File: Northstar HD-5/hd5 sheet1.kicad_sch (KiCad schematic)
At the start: 39 parts, among them Q1 2N3904, U1B1 26LS31, U1C1 74S10, U1D1 74S00, U1E1 50ns_Delay, U1F1 74S04, U1K1 LM393, U1L1 7438, U1M1 74LS374, U2D1 74LS175, U2E1 82S129, U2F1 74S174, U2J1 74LS393, U2K1 74LS393, U2L1 2114, U2M1 2114, U3K1 74LS164, U3L1 74LS374, U3M1 74LS166, U4J1 74LS04, U4K1 74LS244, U4L1 74LS244, U4M1 74LS244, U5L1 74LS138, U5M1 74LS138

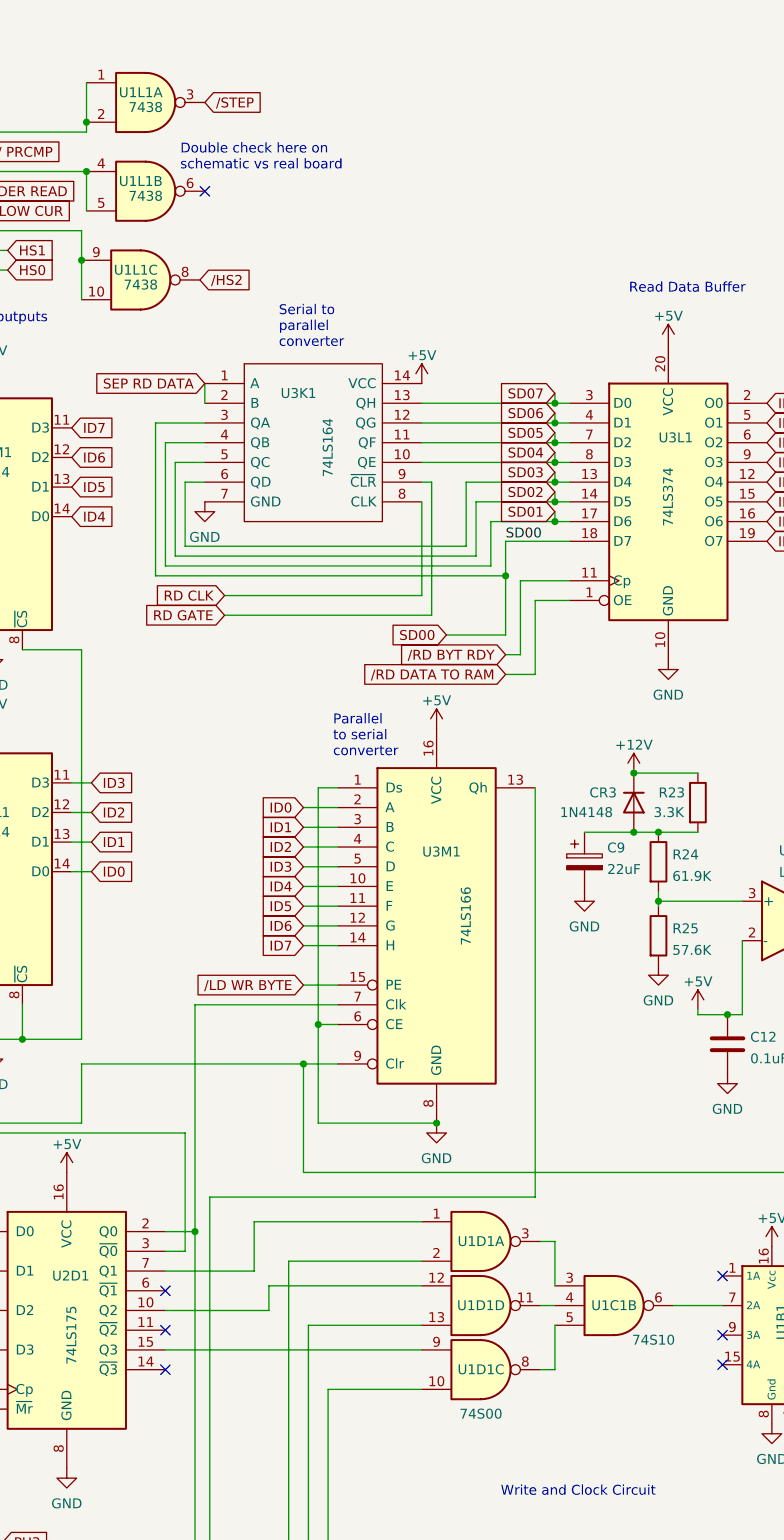
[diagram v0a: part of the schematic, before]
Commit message: small updates to boards
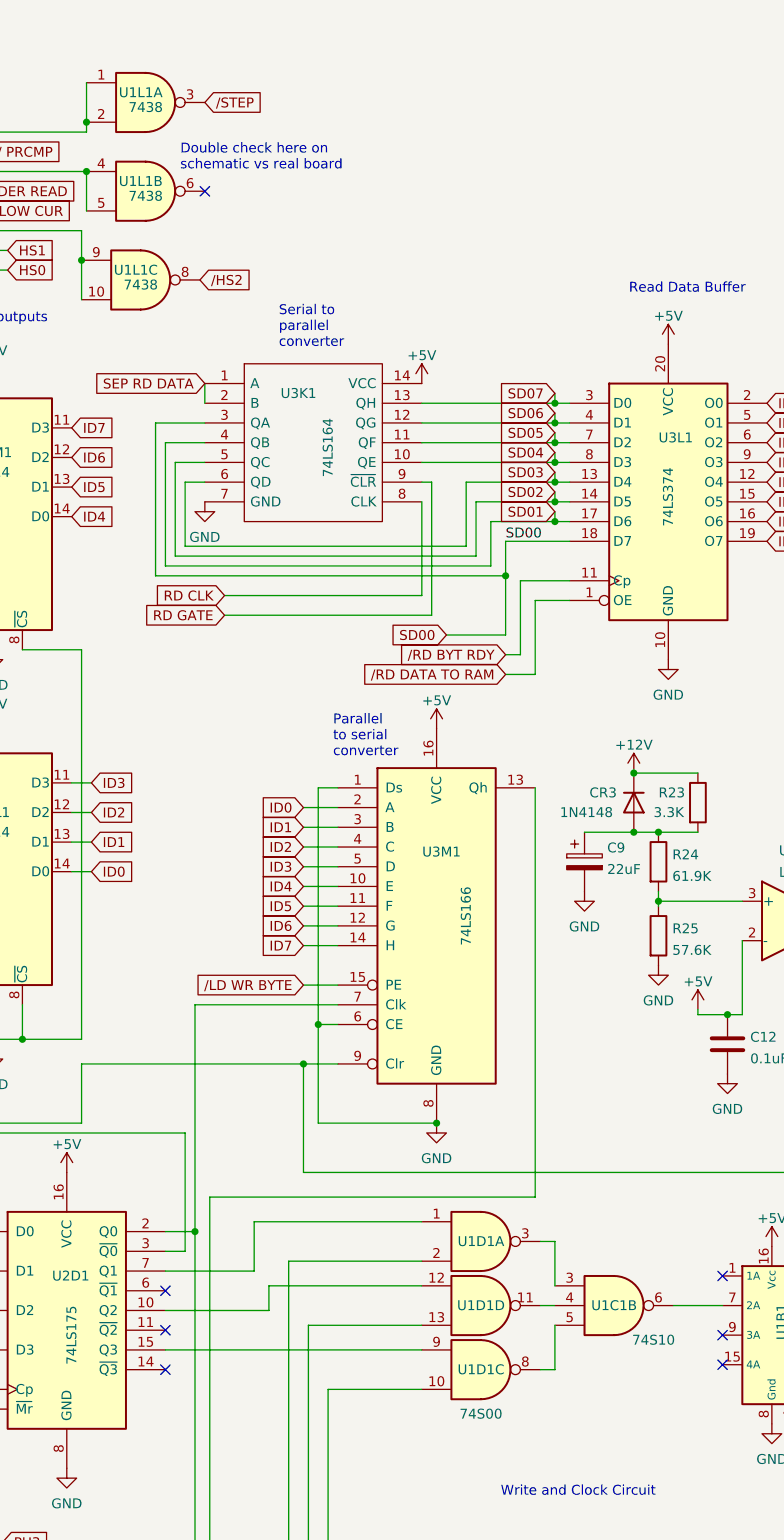
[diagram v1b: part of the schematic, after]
